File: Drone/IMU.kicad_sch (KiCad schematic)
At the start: 6 parts, among them U1 BMX160, U2 BMP388

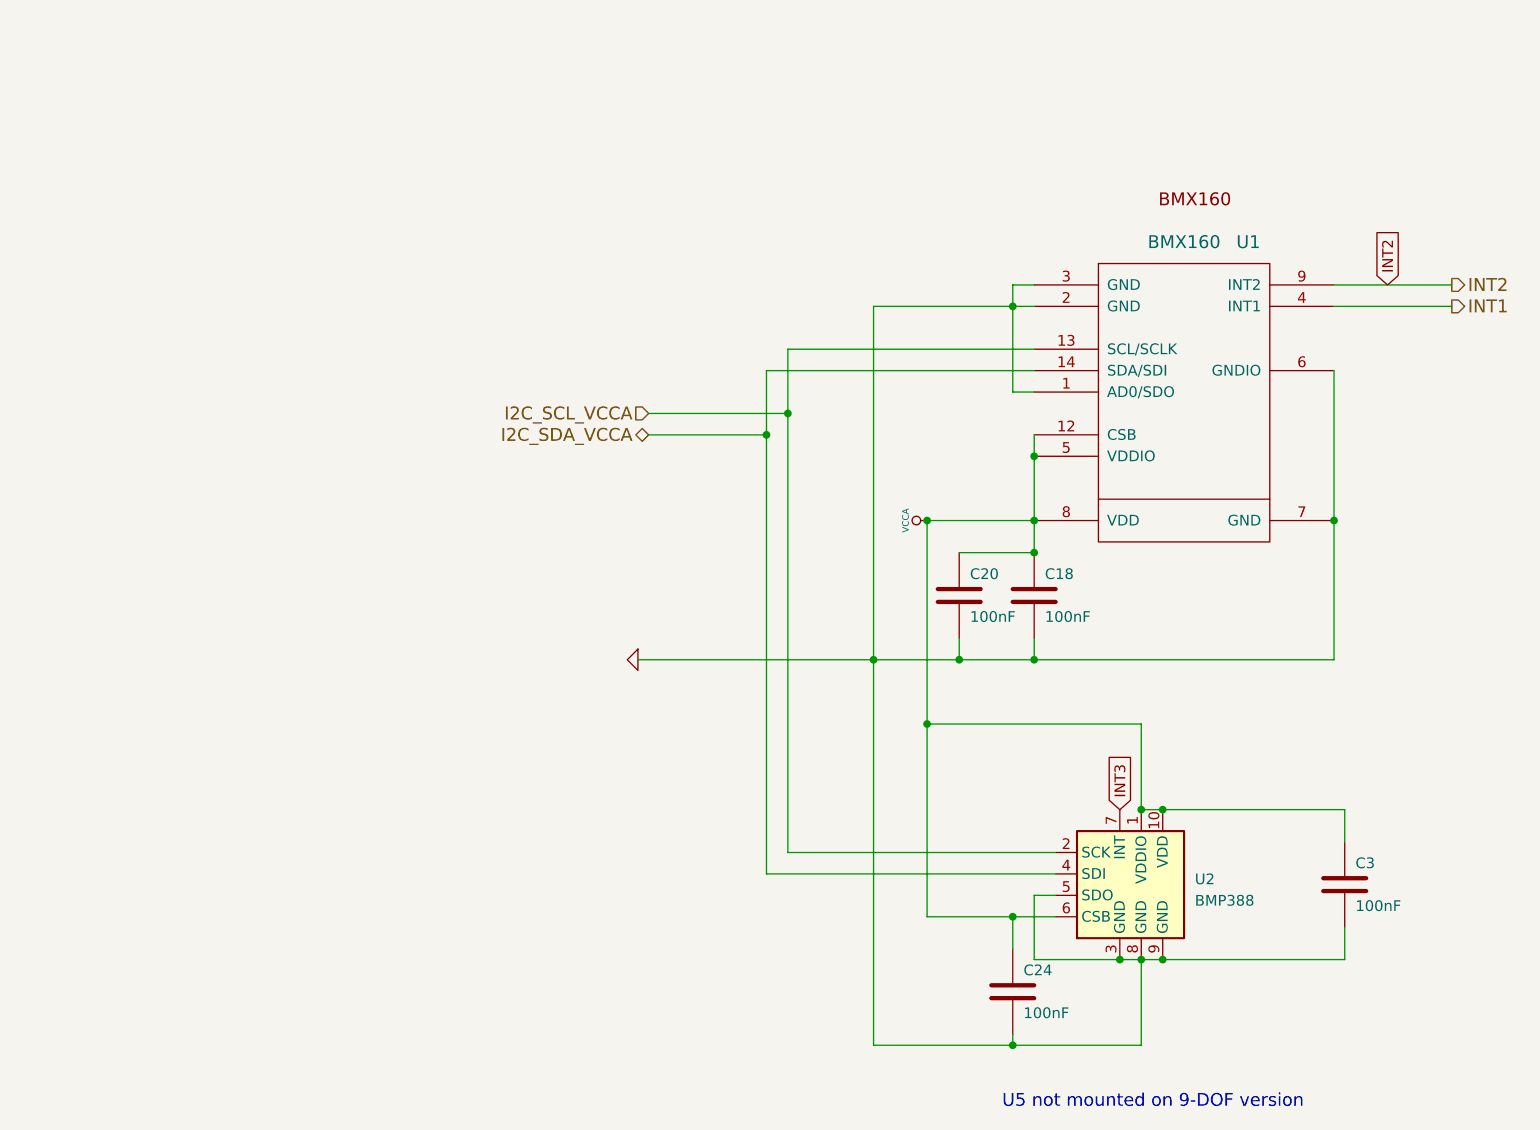
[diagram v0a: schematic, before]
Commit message: save
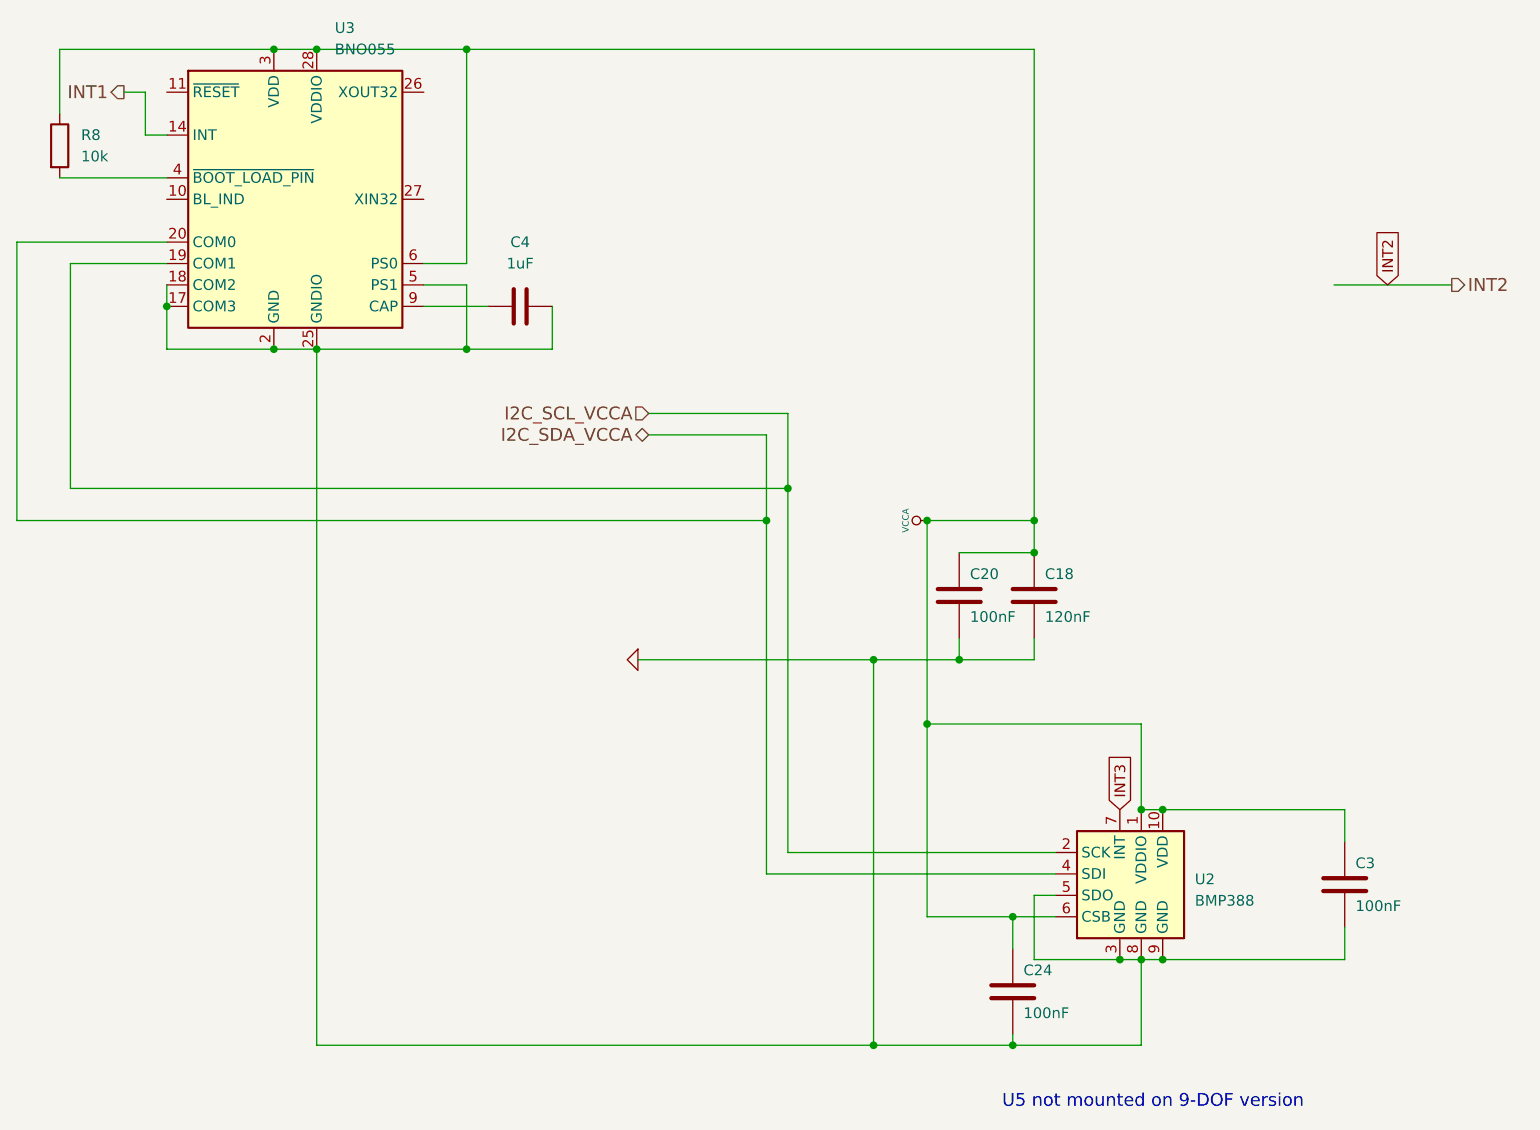
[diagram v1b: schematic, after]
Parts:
- removed U1: BMX160, digikey-footprints:LGA-14L_2.5x3mm__LSM6DS3, symbol Crazyflie-contol-board-rescue:BMX160-SensorMotion
- added C4: 1uF, Capacitor_SMD:C_0603_1608Metric, symbol Device:C
- added R8: 10k, Resistor_SMD:R_0603_1608Metric, symbol Device:R
- added U3: BNO055, Package_LGA:LGA-28_5.2x3.8mm_P0.5mm, symbol Sensor_Motion:BNO055
- C18: value 100nF -> 120nF
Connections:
- net GND: now also C4.2, U3.17 (COM3), U3.18 (COM2), U3.2 (GND), U3.25 (GNDIO), U3.5 (PS1)
- net I2C_SCL_VCCA: now also U3.19 (COM1)
- net I2C_SDA_VCCA: now also U3.20 (COM0)
- net INT1: now also U3.14 (INT)
- net VCCA: now also R8.1, U3.28 (VDDIO), U3.3 (VDD), U3.6 (PS0)
- new net: C4.1, U3.9 (CAP)
- new net: R8.2, U3.4 (~{BOOT_LOAD_PIN})
